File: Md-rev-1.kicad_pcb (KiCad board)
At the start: 2 copper layers, 71.1 x 71.1 mm, 24 parts, among them CN1 JSTPH, J1 USB_C_Receptacle_USB2.0, J2 AudioJack4_SwitchTR1, U1 MCP73831-2-OT, U2 MAX9814

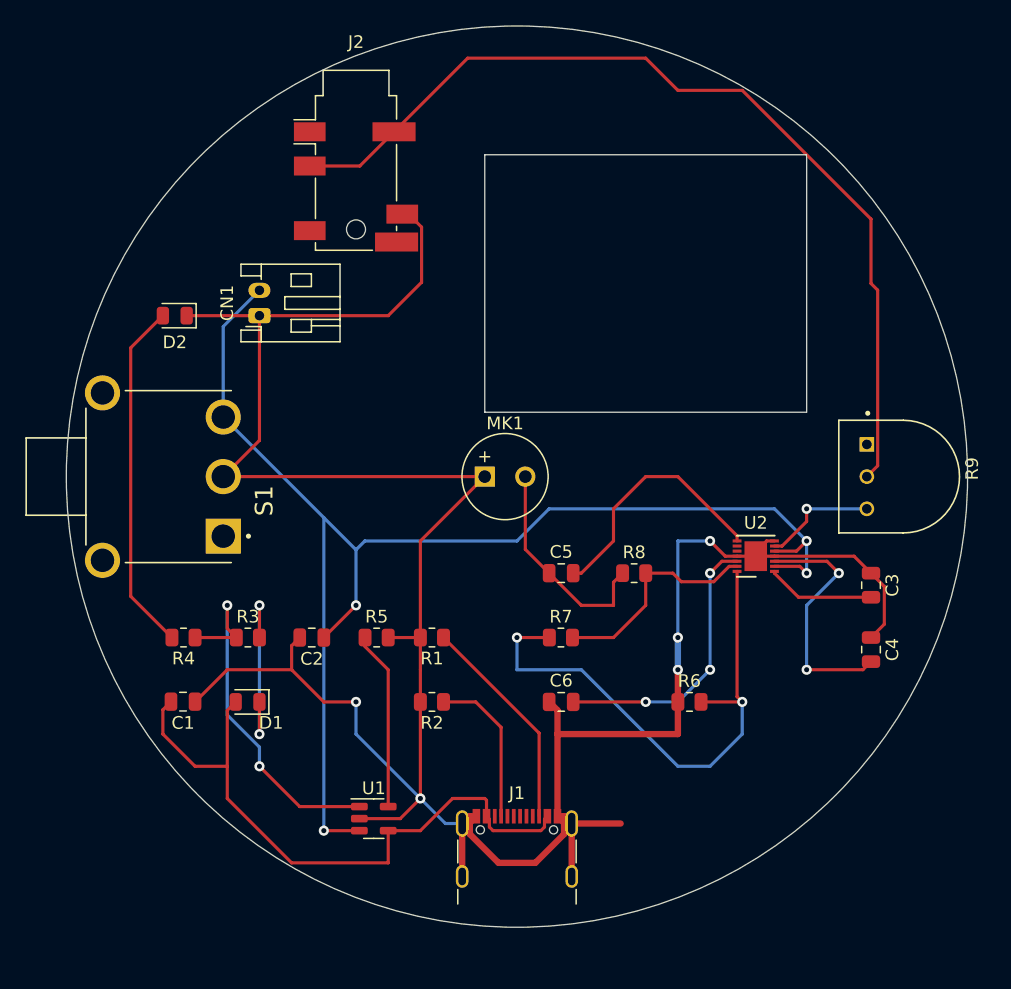
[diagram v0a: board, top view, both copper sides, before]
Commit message: Pushing changes to main
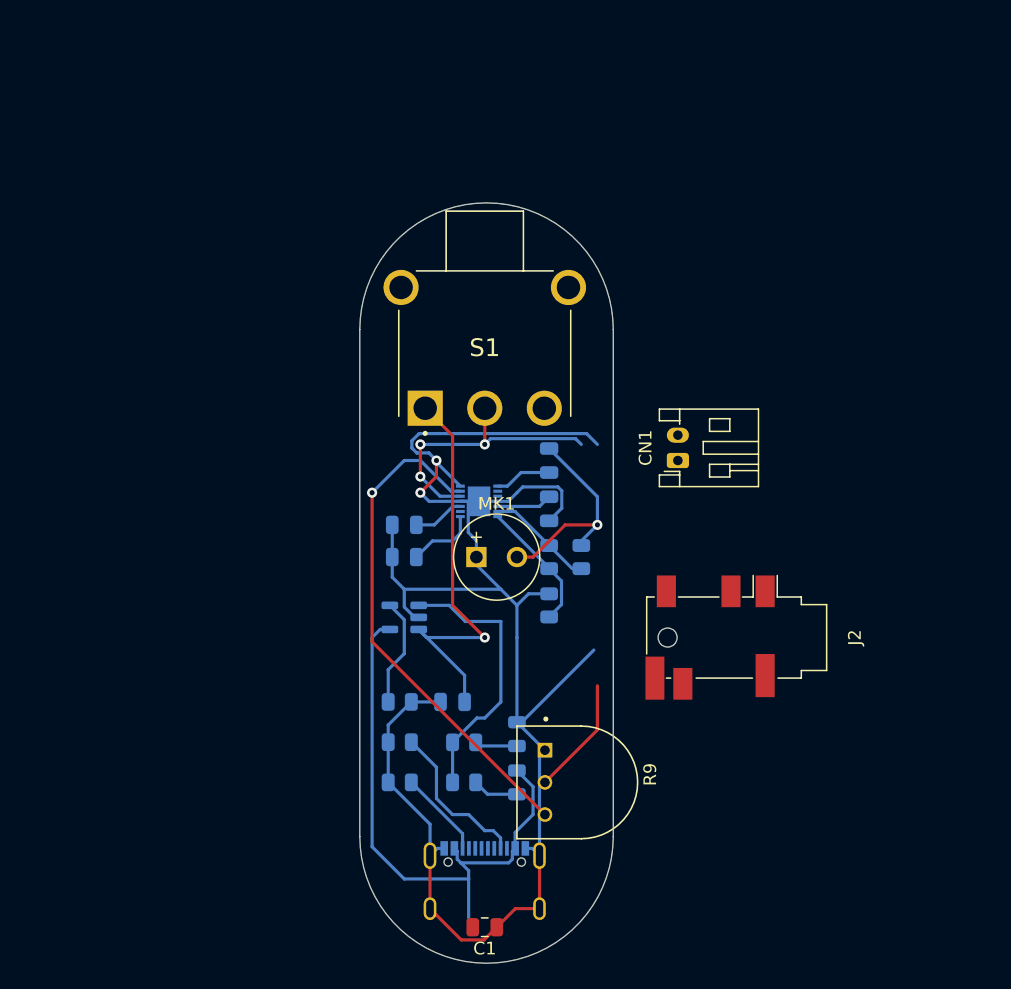
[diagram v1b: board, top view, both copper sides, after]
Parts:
- C2, C3, C4, C5, C6, D1, D2, J1, R1, R2, R3, R4, R5, R6, R7, R8, U1, U2: moved to B.Cu
- moved J2 45.2 mm to (167.6, 114.3), turned to -90 degrees
- moved D2 42.7 mm to (152.4, 121.9), turned to -90 degrees
- moved C4 38.1 mm to (143.5, 105.4), turned to 0 degrees
- moved C3 36.9 mm to (143.5, 108.0), turned to 0 degrees
- moved R9 35.0 mm to (157.5, 125.7)
- moved CN1 34.9 mm to (165.1, 100.3)
- moved C1 29.7 mm to (149.9, 137.2)
- moved S1 27.4 mm to (149.9, 91.4), turned to 0 degrees
- moved R4 23.6 mm to (148.2, 122.6), turned to 0 degrees
- moved U2 22.3 mm to (149.4, 103.6), turned to 0 degrees
- moved D1 22.2 mm to (152.4, 125.7), turned to 90 degrees
- moved R3 20.5 mm to (148.2, 125.7)
- moved U1 16.1 mm to (143.5, 112.7), turned to 180 degrees
- moved C6 15.3 mm to (154.9, 104.1), turned to 90 degrees
- moved R6 13.4 mm to (154.9, 111.8), turned to -90 degrees
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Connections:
- C2 pad 1: /VBAT -> Net-(U1-V_{BAT})
- S1 pad 1: unconnected-(S1-Pad1) -> Net-(U1-V_{BAT})
- S1 pad 2: GND -> /VBAT
- S1 pad 3: /VBAT -> unconnected-(S1-Pad3)
- U1 pad 3: /VBAT -> Net-(U1-V_{BAT})
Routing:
- net /VBAT: track 107.6 -> 22.3 mm, vias 4 -> 3
- net GND: track 213.4 -> 135.5 mm, vias 5 -> 2
- net Net-(J2-PadR1): track 74.0 -> 9.33 mm
- net Net-(U2-TH): track 43.4 -> 10.4 mm, vias 2 -> 0
- net Net-(U1-V_{BAT}): track 0.00 -> 32.7 mm, vias 0 -> 1
- net /OUTPUT: track 9.09 -> 40.1 mm
- net Net-(D2-A): track 27.8 -> 3.44 mm
- net Net-(U2-BIAS): track 22.0 -> 4.37 mm, vias 3 -> 0
- net Net-(U2-MICIN): track 19.9 -> 4.50 mm
- net Net-(U2-CG): track 19.5 -> 4.08 mm, vias 2 -> 0
- net Net-(D1-K): track 15.2 -> 3.64 mm, vias 2 -> 0
- net Net-(J1-CC2): track 17.2 -> 6.89 mm
- net Net-(U2-MICBIAS): track 17.4 -> 9.02 mm
- net Net-(U1-STAT): track 29.0 -> 21.8 mm, vias 2 -> 0
- net Net-(U1-PROG): track 14.1 -> 8.88 mm
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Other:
- board size 71.1 x 71.1 mm -> 20 x 60 mm
